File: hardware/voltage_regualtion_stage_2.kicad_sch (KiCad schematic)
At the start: 22 parts, among them Q3 PMOS, Q5 MUN5334DW1, U15 CPC1907B, U5 TSB712, U6 TMCS1108

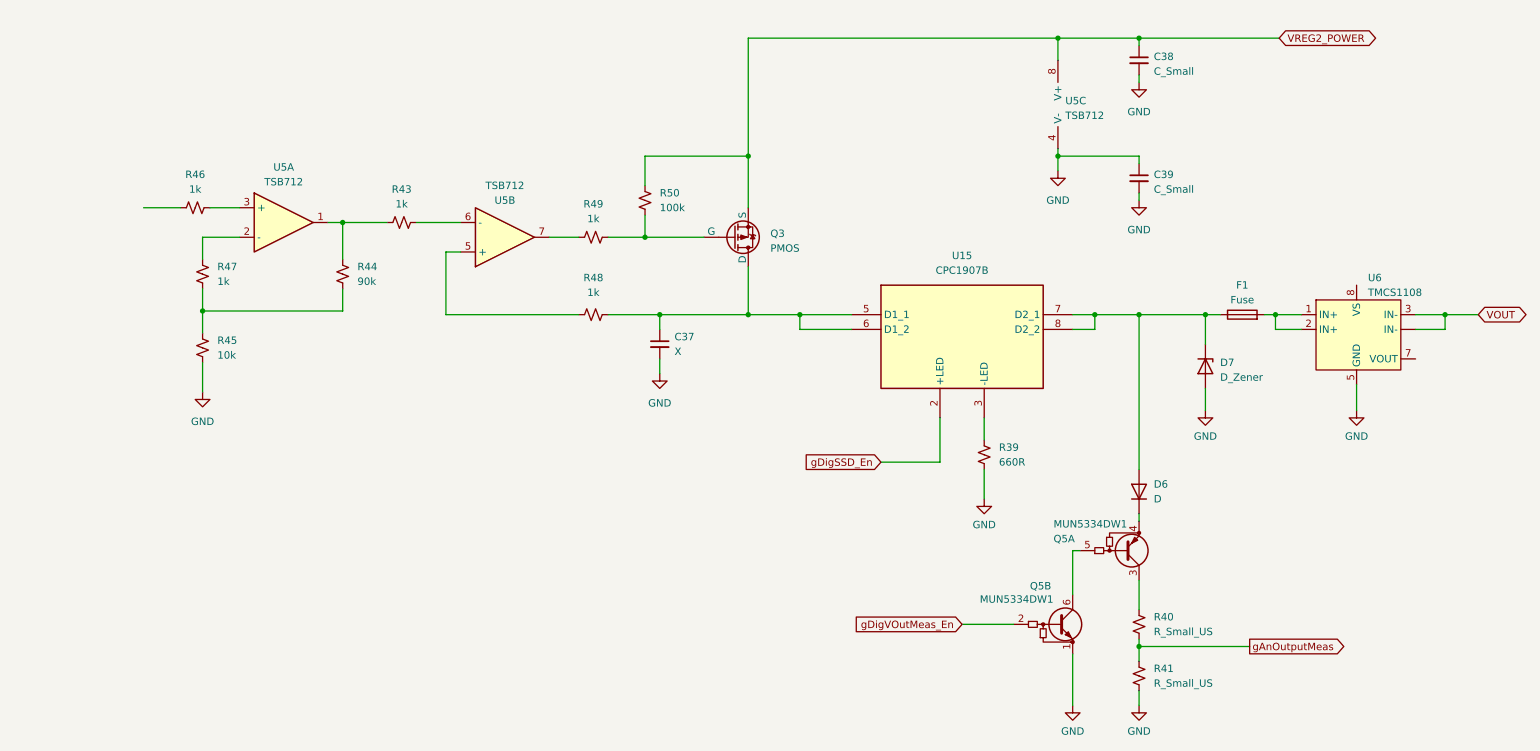
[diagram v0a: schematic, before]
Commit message: Saving prior to changing project structure
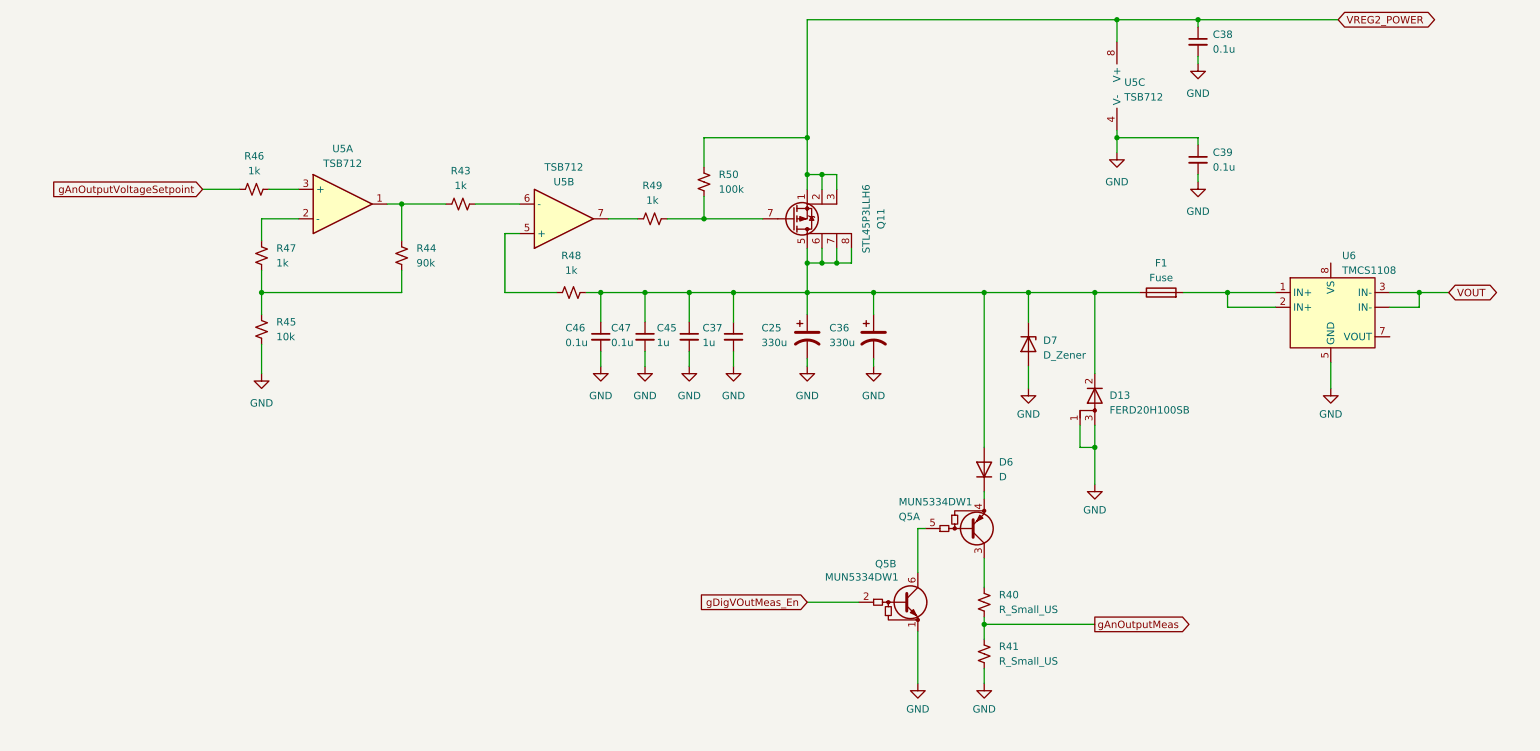
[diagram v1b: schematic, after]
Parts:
- removed Q3: PMOS, symbol Simulation_SPICE:PMOS
- removed R39: 660R, symbol Device:R_Small_US
- removed U15: CPC1907B, Daniel_Solid-State-Relay:CPC1907B, symbol Daniel_Solid-State-Relay:CPC1907B
- added C25, C36: 330u, symbol Device:C_Polarized_US
- added C45: 1u, symbol Device:C_Small
- added C46, C47: 0.1u, symbol Device:C_Small
- added D13: FERD20H100SB, symbol Daniel_Diode:D_AKA
- added Q11: STL45P3LLH6, Daniel_xMOS:PowerFLAT 5x6, symbol Daniel_PMOS:Q_PMOS_DGS
- C37: value X -> 1u
- C38, C39: value C_Small -> 0.1u
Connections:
- net GND: now also C25.2, C36.2, C45.2, C46.2, C47.2, D13.1 (A), D13.3 (A)
- net VREG2_POWER: now also Q11.1 (S), Q11.2 (D), Q11.3 (D)
- net at D6.2 (A), D7.1 (K), F1.1: now also C37.1, R48.1, C25.1, C36.1, C45.1, C46.1, C47.1, D13.2 (K), Q11.5 (D), Q11.6 (D), Q11.7 (G), Q11.8 (D)
- net at R49.2, R50.1: now also Q11.7 (G)
- net gAnOutputVoltageSetpoint: now reaches R46.1
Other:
- moved on the sheet: C37, C38, C39, D6, D7, F1, Q5A, Q5B, R40, R41, R43, R44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
